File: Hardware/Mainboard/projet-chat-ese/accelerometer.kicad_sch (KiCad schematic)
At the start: 4 parts, among them U3 ADXL343BCCZ-RL

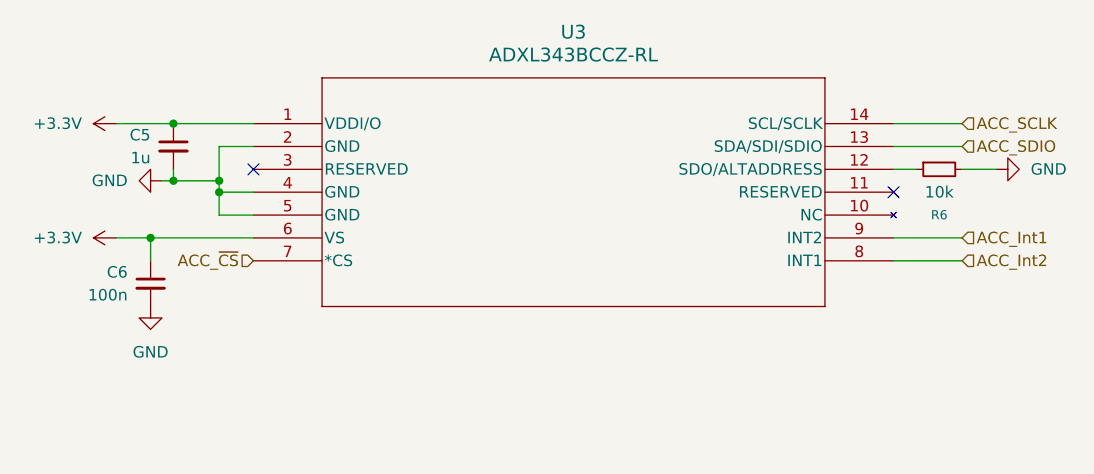
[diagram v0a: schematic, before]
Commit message: [Update] PCB
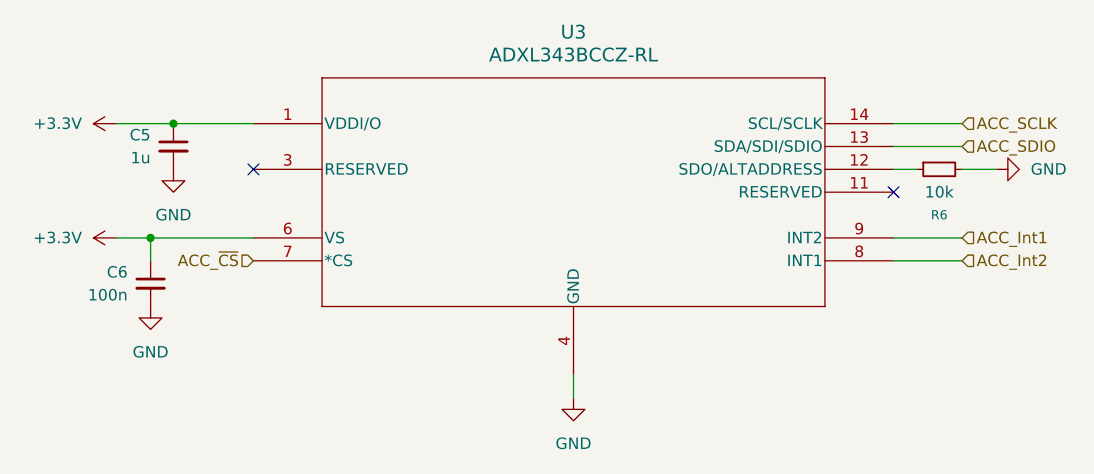
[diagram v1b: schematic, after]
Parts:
- U3: footprint LGA_CC-14-1_ADI -> Custom:LGA_CC-14-1_ADI
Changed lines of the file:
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@@
-	)
-	(junction
-		(at 102.87 95.25)
-		(diameter 0)
-		(color 0 0 0 0)
 	)
 	(junction
@@
 		(color 0 0 0 0)
 	)
-	(junction
-		(at 102.87 93.98)
-		(diameter 0)
-		(color 0 0 0 0)
-	)
-	(junction
-		(at 97.79 93.98)
-		(diameter 0)
-		(color 0 0 0 0)
+	(no_connect
+		(at 177.8 95.25)
 	)
 	(no_connect
 		(at 106.68 92.71)
 	)
-	(no_connect
-		(at 177.8 95.25)
-	)
-	(wire
-		(pts
-			(xy 102.87 93.98) (xy 102.87 95.25)
-		)
-		(stroke
-			(width 0)
-			(type default)
-		)
-	)
 	(wire
 		(pts
@@
 	(wire
 		(pts
-			(xy 96.52 93.98) (xy 97.79 93.98)
-		)
-		(stroke
-			(width 0)
-			(type default)
-		)
-	)
-	(wire
-		(pts
-			(xy 102.87 90.17) (xy 102.87 93.98)
-		)
-		(stroke
-			(width 0)
-			(type default)
-		)
-	)
-	(wire
-		(pts
 			(xy 91.44 100.33) (xy 95.25 100.33)
 		)
@@
 	(wire
 		(pts
-			(xy 97.79 93.98) (xy 102.87 93.98)
-		)
-		(stroke
-			(width 0)
-			(type default)
-		)
-	)
-	(wire
-		(pts
-			(xy 102.87 95.25) (xy 102.87 97.79)
-		)
-		(stroke
-			(width 0)
-			(type default)
-		)
-	)
-	(wire
-		(pts
 			(xy 185.42 87.63) (xy 177.8 87.63)
 		)
@@
 	(wire
 		(pts
-			(xy 102.87 97.79) (xy 106.68 97.79)
-		)
-		(stroke
-			(width 0)
-			(type default)
-		)
-	)
-	(wire
-		(pts
-			(xy 102.87 95.25) (xy 106.68 95.25)
-		)
-		(stroke
-			(width 0)
-			(type default)
-		)
-	)
-	(wire
-		(pts
 			(xy 91.44 87.63) (xy 97.79 87.63)
 		)
@@
 	(wire
 		(pts
-			(xy 106.68 90.17) (xy 102.87 90.17)
-		)
-		(stroke
-			(width 0)
-			(type default)
-		)
-	)
-	(wire
-		(pts
-			(xy 97.79 92.71) (xy 97.79 93.98)
+			(xy 142.24 115.57) (xy 142.24 118.11)
 		)
 		(stroke
@@
 	(symbol
 		(lib_id "power:GND")
-		(at 96.52 93.98 270)
+		(at 142.24 118.11 0)
+		(unit 1)
+		(exclude_from_sim no)
+		(in_bom yes)
+		(on_board yes)
+		(dnp no)
+		(fields_autoplaced yes)
+		(property "Reference" "#PWR0301"
+			(at 142.24 124.46 0)
+			(effects
+				(font
+					(size 1.27 1.27)
+				)
+				(hide yes)
+			)
+		)
+		(property "Value" "GND"
+			(at 142.24 123.19 0)
+			(effects
+				(font
+					(size 1.27 1.27)
+				)
+			)
+		)
+		(property "Footprint" ""
+			(at 142.24 118.11 0)
+			(effects
+				(font
+					(size 1.27 1.27)
+				)
+				(hide yes)
+			)
+		)
+		(property "Datasheet" ""
+			(at 142.24 118.11 0)
+			(effects
+				(font
+					(size 1.27 1.27)
+				)
+				(hide yes)
+			)
+		)
+		(property "Description" "Power symbol creates a global label with name \"GND\" , ground"
+			(at 142.24 118.11 0)
+			(effects
+				(font
+					(size 1.27 1.27)
+				)
+				(hide yes)
+			)
+		)
+		(pin "1"
+		)
+		(instances
+			(project "projet-chat-ese"
+				(path "/3d65b2f4-4354-4e18-9b77-809d2b1122a1/64873241-b38d-455e-8523-56dba9a4e972"
+					(reference "#PWR0301")
+					(unit 1)
+				)
+			)
+		)
+	)
+	(symbol
+		(lib_id "power:GND")
+		(at 97.79 92.71 0)
 		(unit 1)
 		(exclude_from_sim no)
@@
 		(fields_autoplaced yes)
 		(property "Reference" "#PWR017"
-			(at 90.17 93.98 0)
+			(at 97.79 99.06 0)
 			(effects
 				(font
@@
 		)
 		(property "Value" "GND"
-			(at 92.71 93.9799 90)
-			(effects
-				(font
-					(size 1.27 1.27)
-				)
-				(justify right)
+			(at 97.79 97.79 0)
+			(effects
+				(font
+					(size 1.27 1.27)
+				)
 			)
 		)
 		(property "Footprint" ""
-			(at 96.52 93.98 0)
+			(at 97.79 92.71 0)
 			(effects
 				(font
@@
 		)
 		(property "Datasheet" ""
-			(at 96.52 93.98 0)
+			(at 97.79 92.71 0)
 			(effects
 				(font
@@
 		)
 		(property "Description" "Power symbol creates a global label with name \"GND\" , ground"
-			(at 96.52 93.98 0)
+			(at 97.79 92.71 0)
 			(effects
 				(font
@@
 			)
 		)
-		(property "Footprint" "LGA_CC-14-1_ADI"
+		(property "Footprint" "Custom:LGA_CC-14-1_ADI"
 			(at 106.68 87.63 0)
 			(effects
